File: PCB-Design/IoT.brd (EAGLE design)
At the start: 59.7 x 51.7 mm, 11 parts, among them M2 ARDUINO-NANO-3.0, M3 WIRELESS-NRF24L01

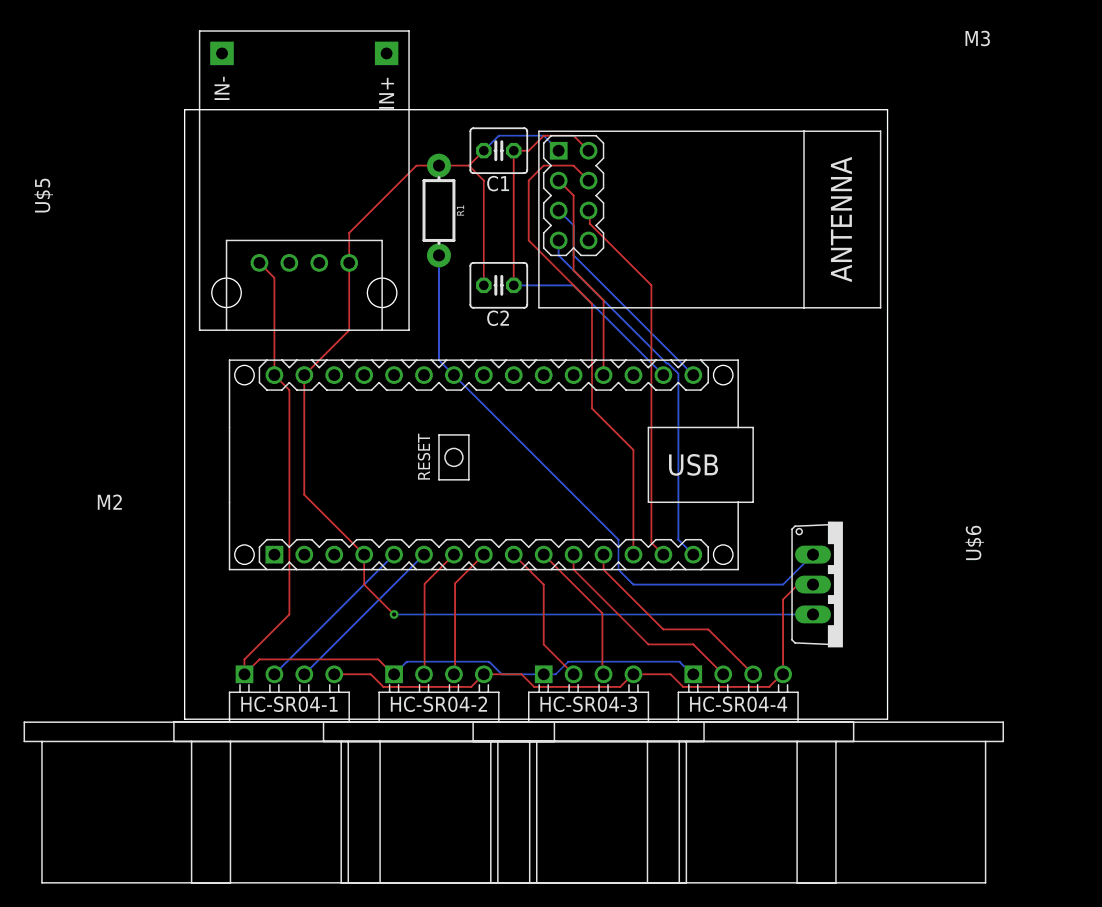
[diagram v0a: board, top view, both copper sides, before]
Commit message: PCB edit
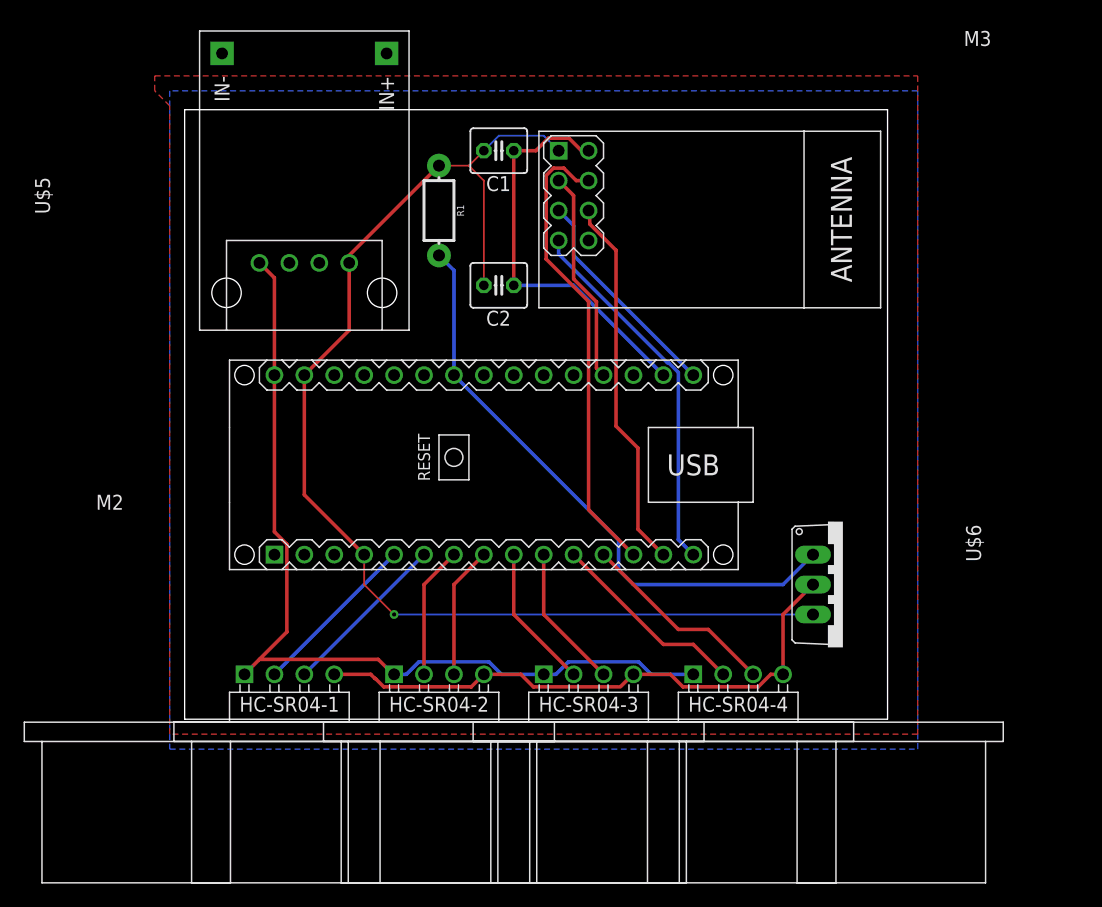
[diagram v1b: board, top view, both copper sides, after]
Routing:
- net N$15: track 41.6 -> 39.6 mm
- net VCC: track 78.5 -> 76.5 mm
- net GND: track 105.4 -> 104.3 mm
- net N$9: track 50.2 -> 49.4 mm
- net N$13: track 17.7 -> 16.9 mm
- net N$12: track 17.7 -> 16.9 mm
- added copper zone on layer 1, net GND
- added copper zone on layer 16, net GND

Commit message: Redone PCB on bottom only
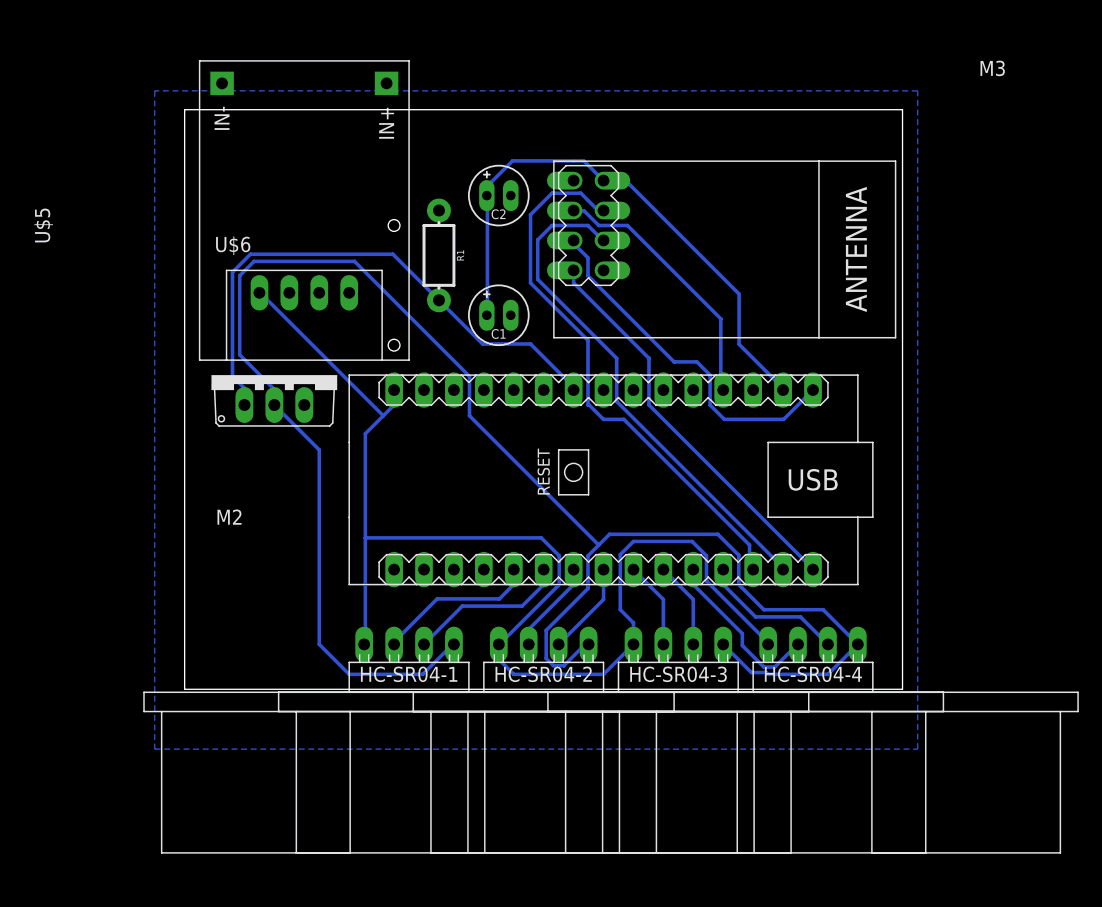
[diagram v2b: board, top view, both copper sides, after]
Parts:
- C1, C2: value (none) -> 10U/35V; device resistor:C025-040X050 -> capacitors-electrolytic:E2-5
- moved U$6 51.4 mm to (5.08, 78.7), turned to 0 degrees
- moved C1 14.0 mm to (24.1, 83.8), turned to 0 degrees
- moved HC-SR04-1 10.5 mm to (16.5, 55.9)
- moved M2 10.2 mm to (33.0, 69.8)
- moved HC-SR04-2 9.25 mm to (27.9, 55.9)
- moved HC-SR04-3 8.03 mm to (39.4, 55.9)
- moved C2 7.62 mm to (24.1, 94.0), turned to 0 degrees
- moved HC-SR04-4 6.84 mm to (50.8, 55.9)
- moved R1 3.81 mm to (19.1, 88.9)
- moved M3 2.84 mm to (43.2, 88.9)
- moved U$5 2.54 mm to (7.62, 92.7)
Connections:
- removed net N$4: C1.1, C2.1, M2.J2.14, M3.2
- new net N$2: C1.+, C2.+, M2.J2.14, M3.2
- net GND: now also C1.-, C2.-; no longer C1.2, C2.2
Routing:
- net GND: track 104.3 -> 0.00 mm, vias 1 -> 0
- net N$9: track 49.4 -> 147.9 mm
- net N$2: track 0.00 -> 47.6 mm
- net N$4: track 34.7 -> 0.00 mm
- net VCC: track 76.5 -> 104.5 mm
- net N$16: track 18.7 -> 30.2 mm
- net N$17: track 31.9 -> 43.2 mm
- net N$15: track 39.6 -> 46.7 mm
- net N$11: track 12.3 -> 7.40 mm
- net N$10: track 12.3 -> 7.40 mm
- net N$1: track 51.1 -> 46.2 mm
- net N$12: track 16.9 -> 12.3 mm
- net N$14: track 18.1 -> 22.5 mm
- net N$8: track 11.2 -> 7.93 mm
- net N$7: track 11.2 -> 7.93 mm
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- removed copper zone on layer 1, net GND
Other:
- board size 59.7 x 51.7 mm -> 60.9 x 49.2 mm
